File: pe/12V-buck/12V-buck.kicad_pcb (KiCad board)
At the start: 2 copper layers, 9 parts, among them U1 TPS563208

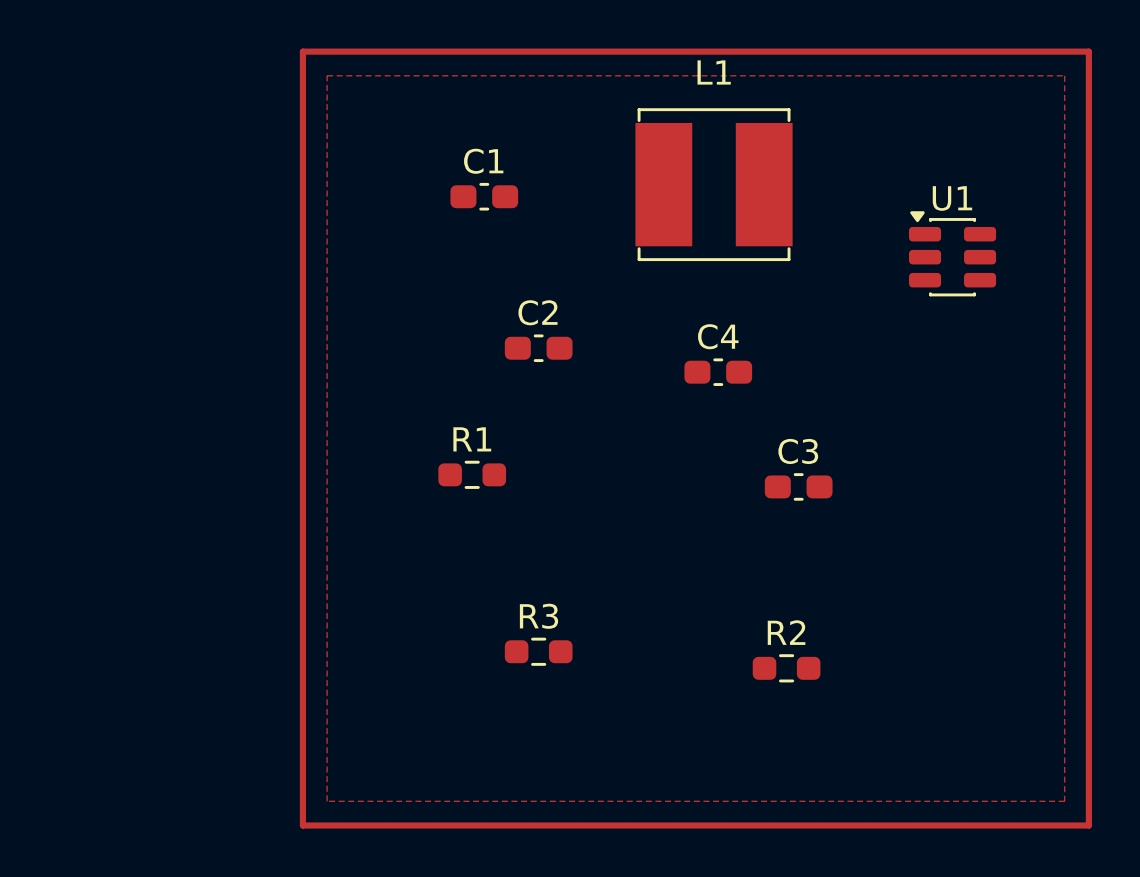
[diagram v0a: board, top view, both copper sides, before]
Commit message: pcb update
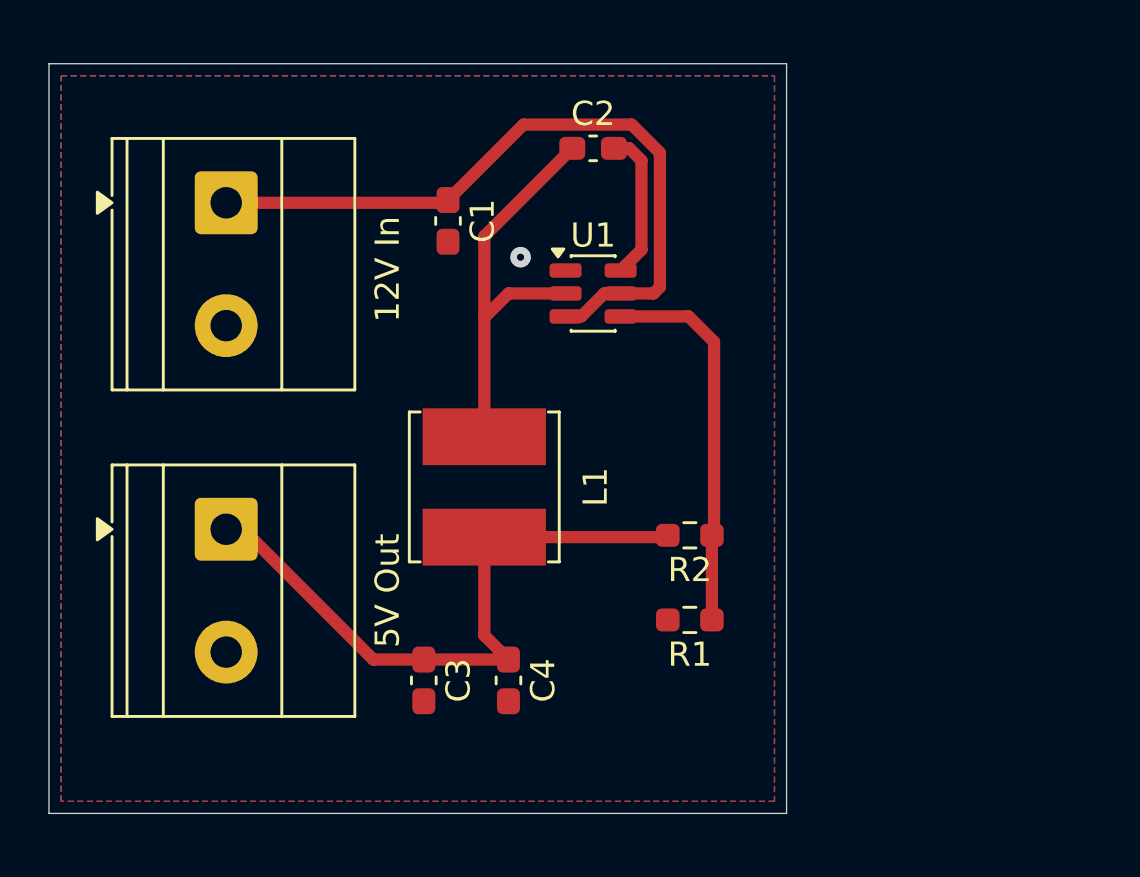
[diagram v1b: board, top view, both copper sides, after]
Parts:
- removed the R1 at (130.0, 96.0)
- added 12V In: 12V, TerminalBlock_Phoenix:TerminalBlock_Phoenix_MKDS-1,5-2-5.08_1x02_P5.08mm_Horizontal, F.Cu at (119.8, 84.8)
- added 5V Out: 5V, TerminalBlock_Phoenix:TerminalBlock_Phoenix_MKDS-1,5-2-5.08_1x02_P5.08mm_Horizontal, F.Cu at (119.8, 98.2)
- moved C3 17.4 mm to (128.0, 104.5), turned to -90 degrees
- moved L1 15.7 mm to (130.5, 96.5), turned to -90 degrees
- moved C4 15.4 mm to (131.5, 104.5), turned to -90 degrees
- moved U1 14.9 mm to (135.0, 88.5)
- moved C2 8.57 mm to (135.0, 82.5)
- moved R2 7.89 mm to (139.0, 98.5), turned to 180 degrees
- moved R1 4.47 mm to (139.0, 102.0), turned to 180 degrees
- moved C1 1.80 mm to (129.0, 85.5), turned to -90 degrees
- renumbered R2 to R1, R3 to R2
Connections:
- U1 pad 5: Net-(U1-EN) -> +12V
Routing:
- net +12V: track 0.00 -> 29.0 mm
- net +5V: track 0.00 -> 26.3 mm
- net Net-(U1-SW): track 0.00 -> 17.2 mm
- net Net-(U1-VFB): track 0.00 -> 15.8 mm
- net Net-(U1-VBST): track 0.00 -> 6.25 mm
- net GND: vias 0 -> 1
- added copper zone on B.Cu, net GND
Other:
- board outline added: 30.5 x 31 mm
